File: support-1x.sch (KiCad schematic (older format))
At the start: 27 parts, among them P1 CONN_01X02, P2 TL431, P3 LM335, Q1 Q_NMOS_GSD, U1 LM358

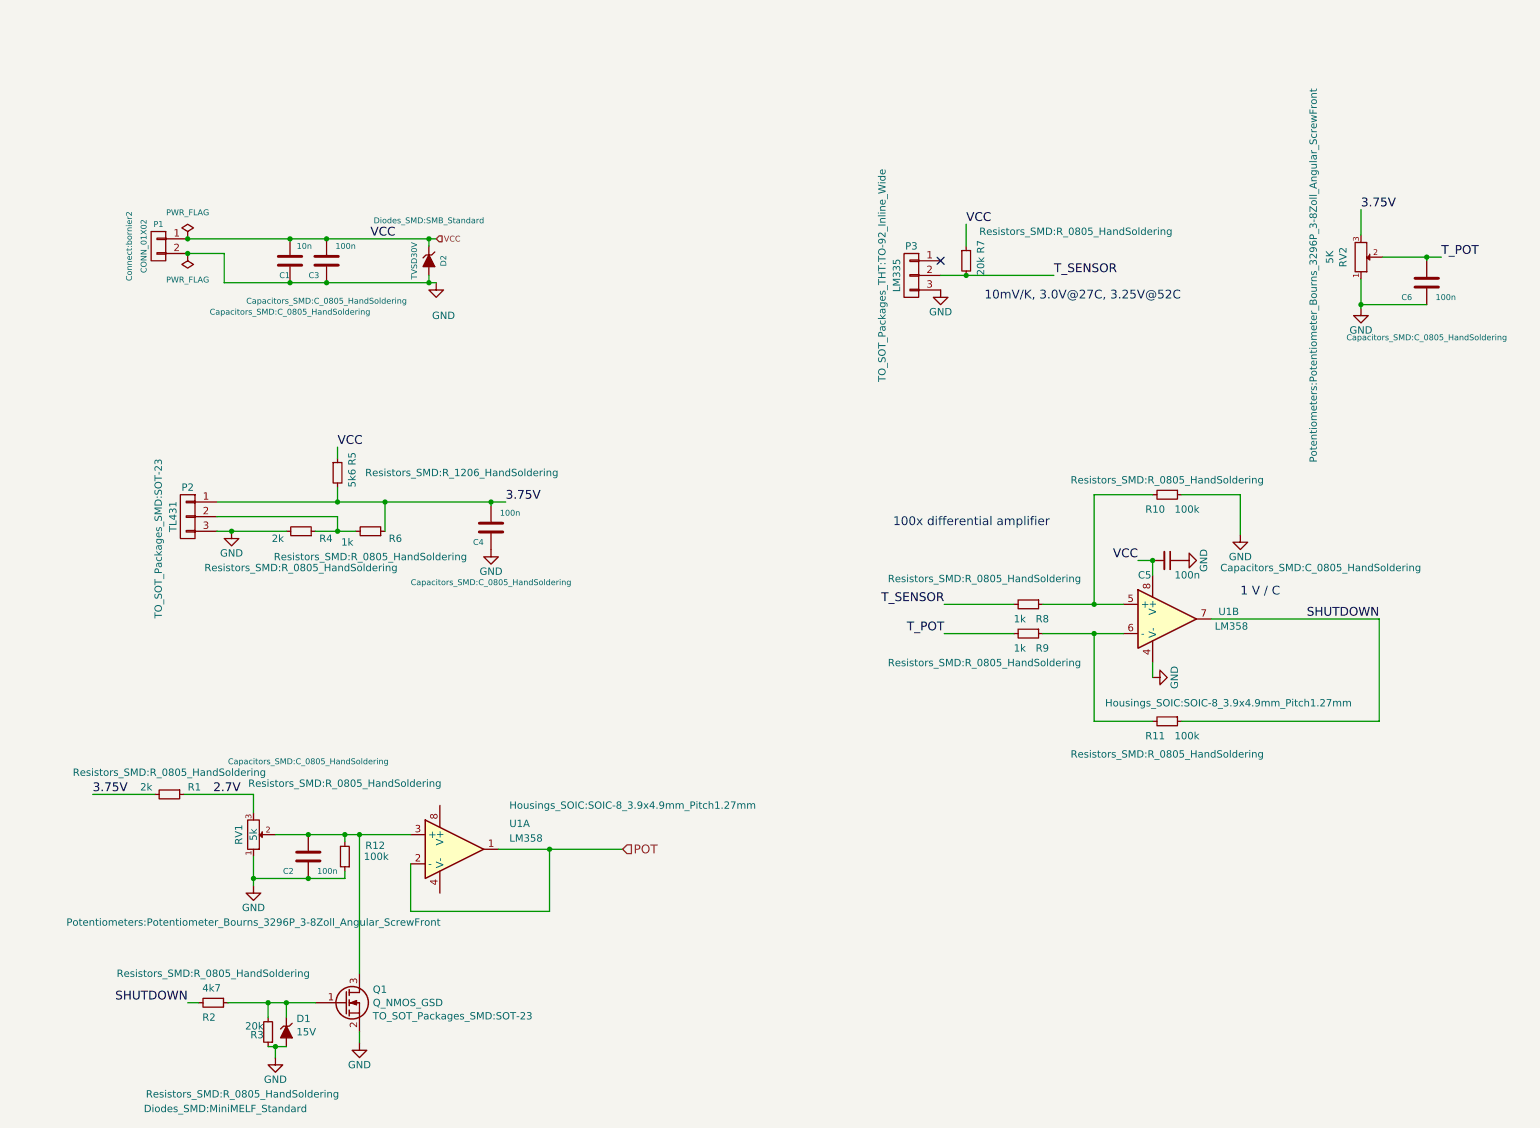
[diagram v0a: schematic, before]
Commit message: Few improvements
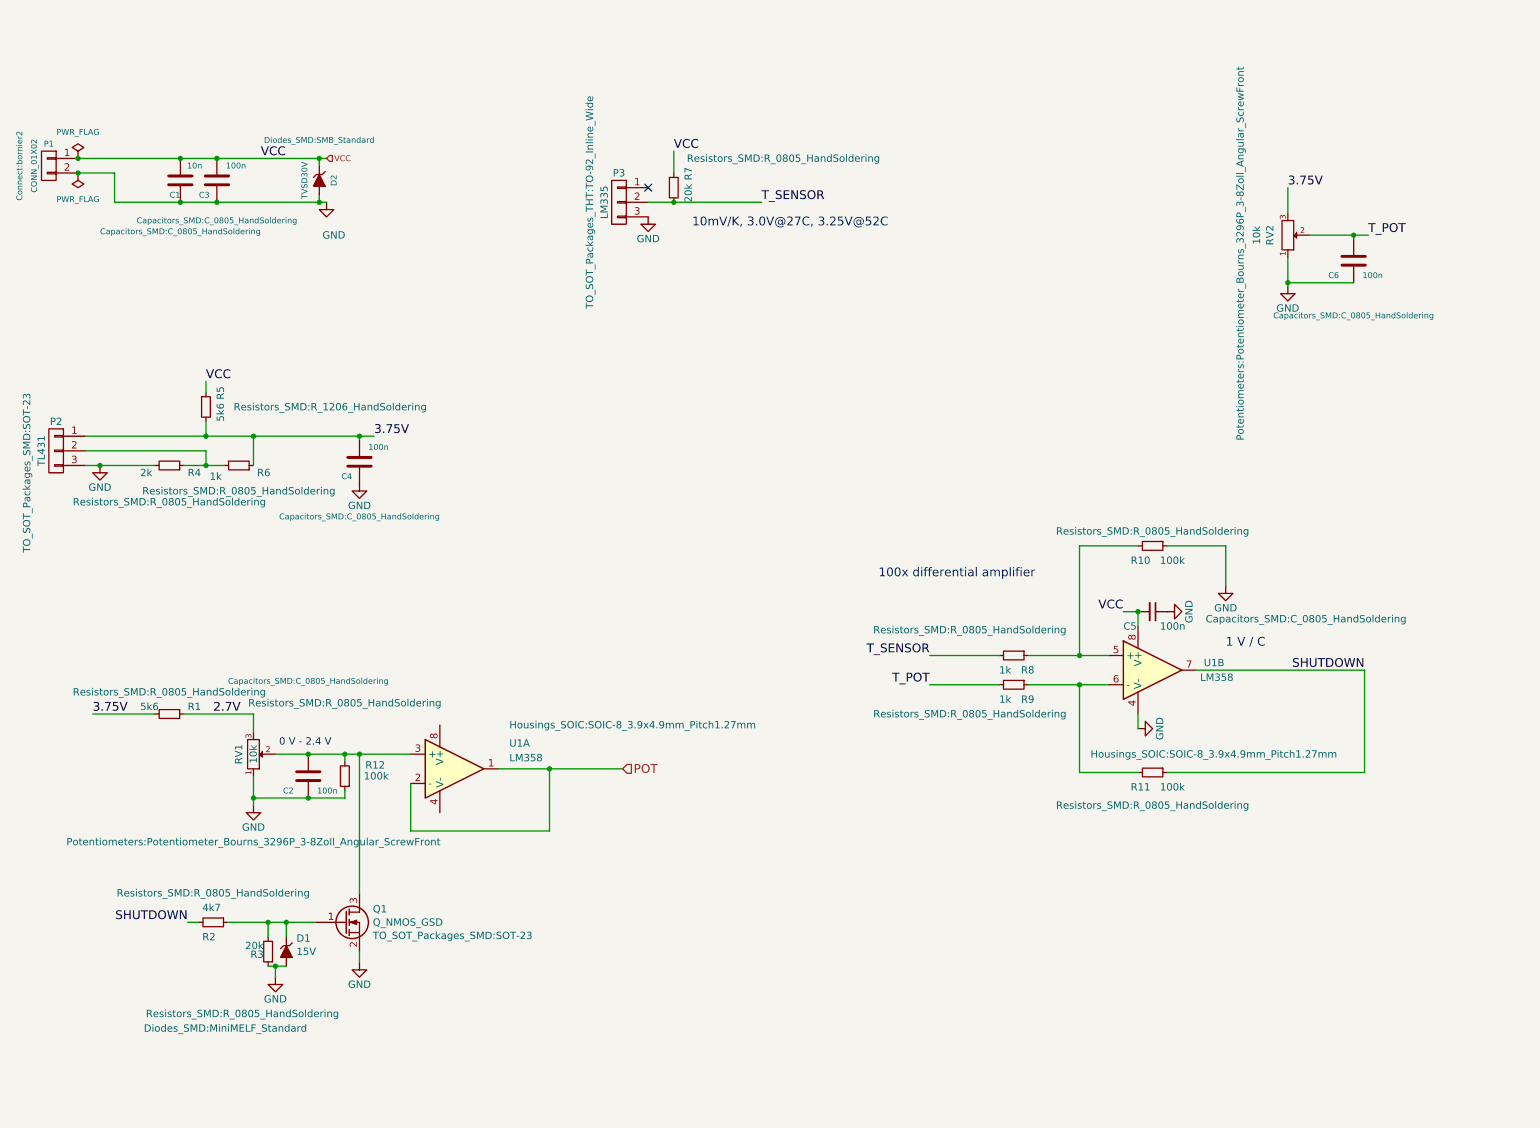
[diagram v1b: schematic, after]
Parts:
- R1: value 2k -> 5k6
- RV1: value 5k -> 10k
- RV2: value 5K -> 10k
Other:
- note added: "0 V - 2.4 V\n"
- moved on the sheet: C1, C2, C3, C4, C5, C6, D1, D2, P1, P2, P3, Q1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
